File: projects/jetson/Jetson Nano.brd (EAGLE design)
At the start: 97.8 x 82.2 mm, 20 parts

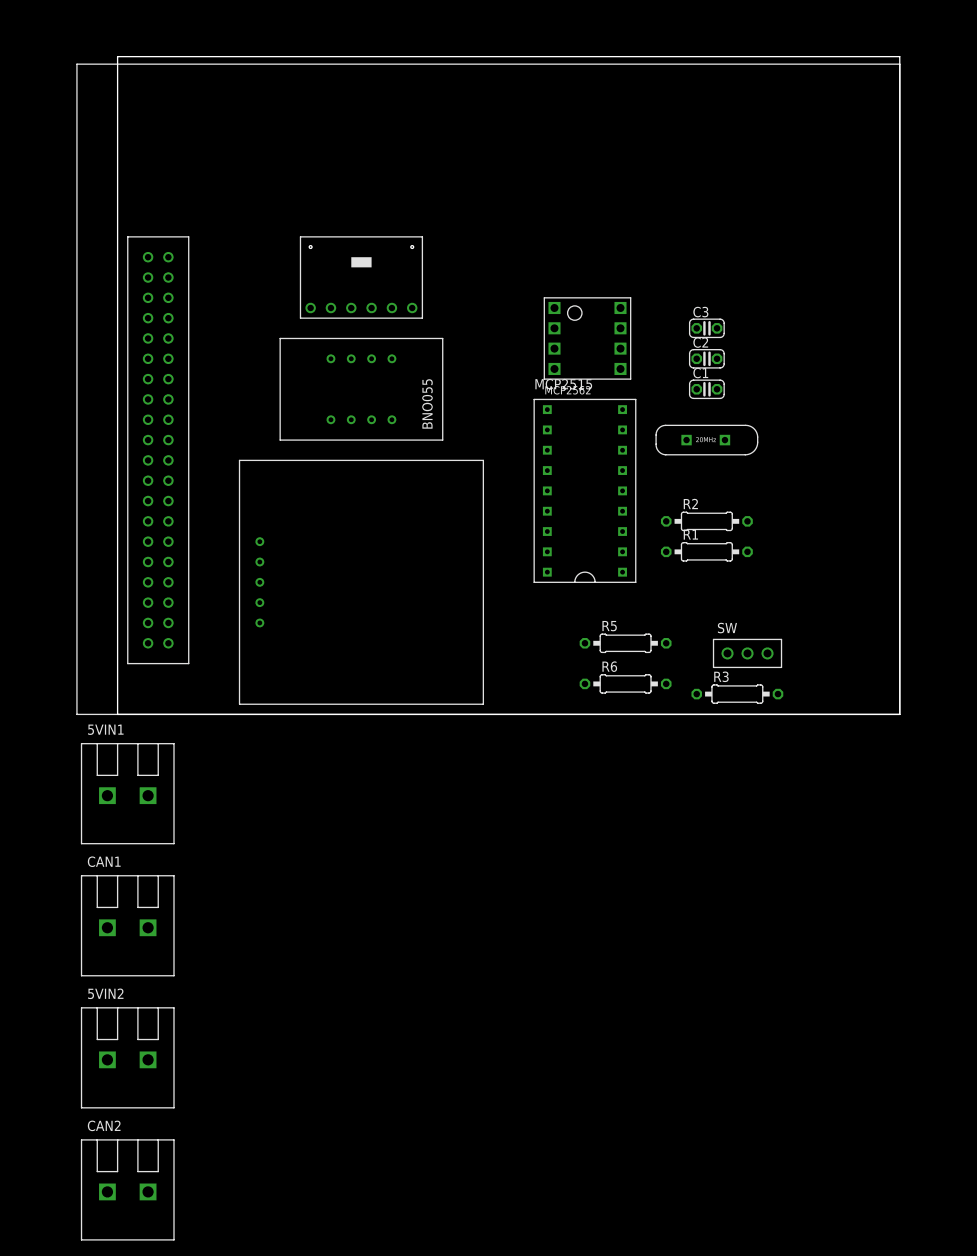
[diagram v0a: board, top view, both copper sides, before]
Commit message: add
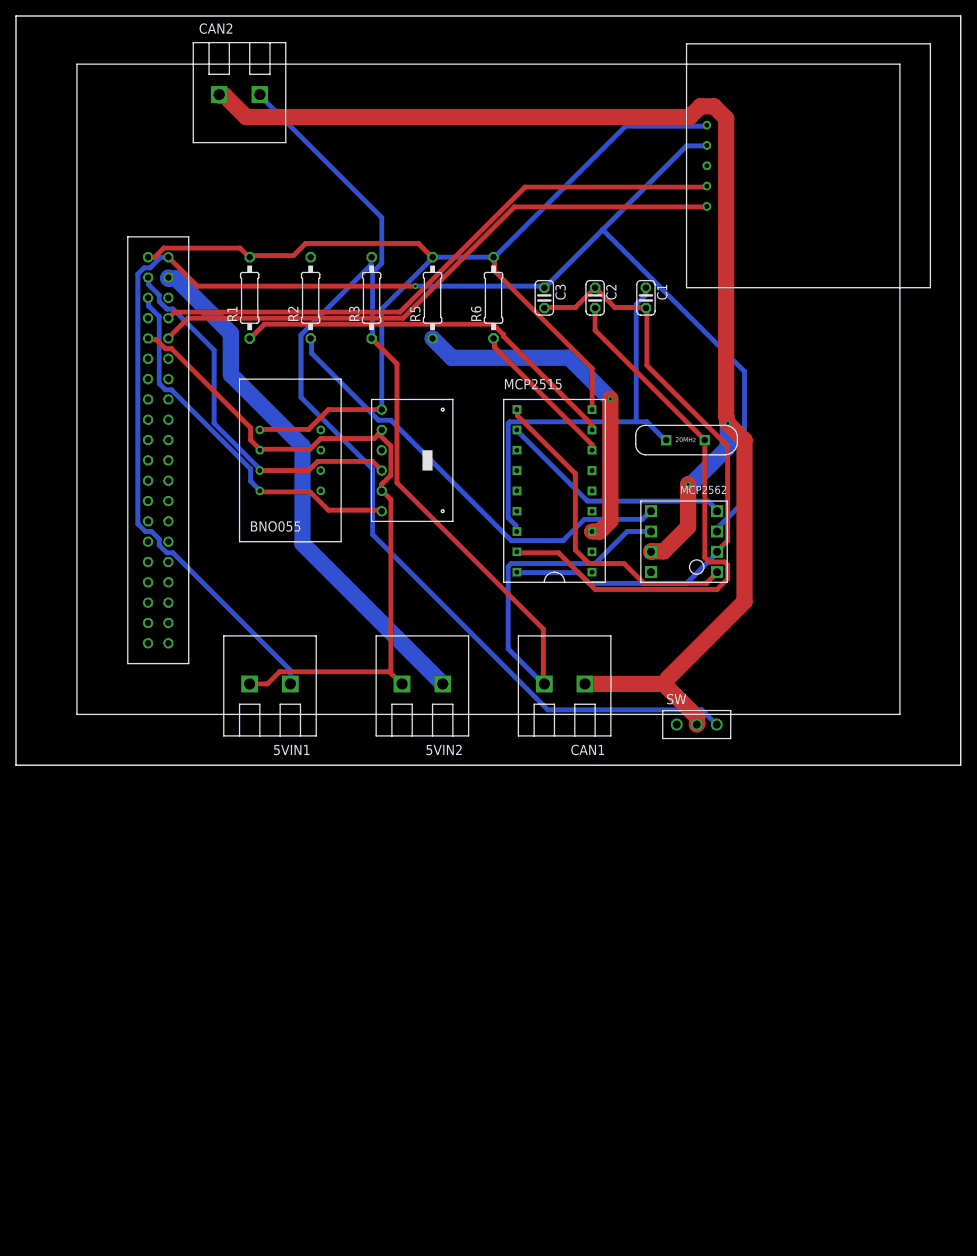
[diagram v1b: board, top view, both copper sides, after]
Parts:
- moved CAN2 137.9 mm to (20.3, 77.5)
- moved U$3 76.4 mm to (78.7, 68.6)
- moved R3 67.4 mm to (36.8, 52.1), turned to 90 degrees
- moved R1 65.4 mm to (21.6, 52.1), turned to 90 degrees
- moved CAN1 62.5 mm to (61.0, 3.81), turned to 180 degrees
- moved 5VIN2 59.7 mm to (43.2, 3.81), turned to 180 degrees
- moved R2 56.9 mm to (29.2, 52.1), turned to 90 degrees
- moved R6 51.0 mm to (52.1, 52.1), turned to 90 degrees
- moved R5 49.5 mm to (44.5, 52.1), turned to 90 degrees
- moved U$4 25.4 mm to (80.0, 26.7), turned to 180 degrees
- moved 5VIN1 22.6 mm to (24.1, 3.81), turned to 180 degrees
- moved C3 20.7 mm to (58.4, 52.1), turned to 270 degrees
- moved C2 15.9 mm to (64.8, 52.1), turned to 270 degrees
- moved U$1 15.3 mm to (38.1, 39.4), turned to 270 degrees
- moved C1 13.7 mm to (71.1, 52.1), turned to 270 degrees
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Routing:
- net +5V: track 0.00 -> 187.5 mm, vias 0 -> 1
- net CAN_H2: track 0.00 -> 179.2 mm, vias 0 -> 2
- net +3V3: track 0.00 -> 141.3 mm
- net N$16: track 0.00 -> 125.8 mm
- net N$15: track 0.00 -> 94.9 mm
- net N$2: track 0.00 -> 88.9 mm
- net V-: track 0.00 -> 77.4 mm
- net N$12: track 0.00 -> 74.2 mm
- net N$11: track 0.00 -> 74.2 mm
- net N$7: track 0.00 -> 70.7 mm
- net 5V_2: track 0.00 -> 65.6 mm
- net N$14: track 0.00 -> 55.5 mm
- net N$5: track 0.00 -> 52.1 mm
- net N$13: track 0.00 -> 49.5 mm
- net N$4: track 0.00 -> 46.8 mm
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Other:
- board size 97.8 x 82.2 mm -> 118.1 x 93.6 mm
